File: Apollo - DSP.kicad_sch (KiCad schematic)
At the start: 27 parts, among them J1 USB_C_Receptacle_USB2.0, U1 NCP115ASN330T2G, U2 USBLC6-2SC6, U3 NCP115ASN330T2G

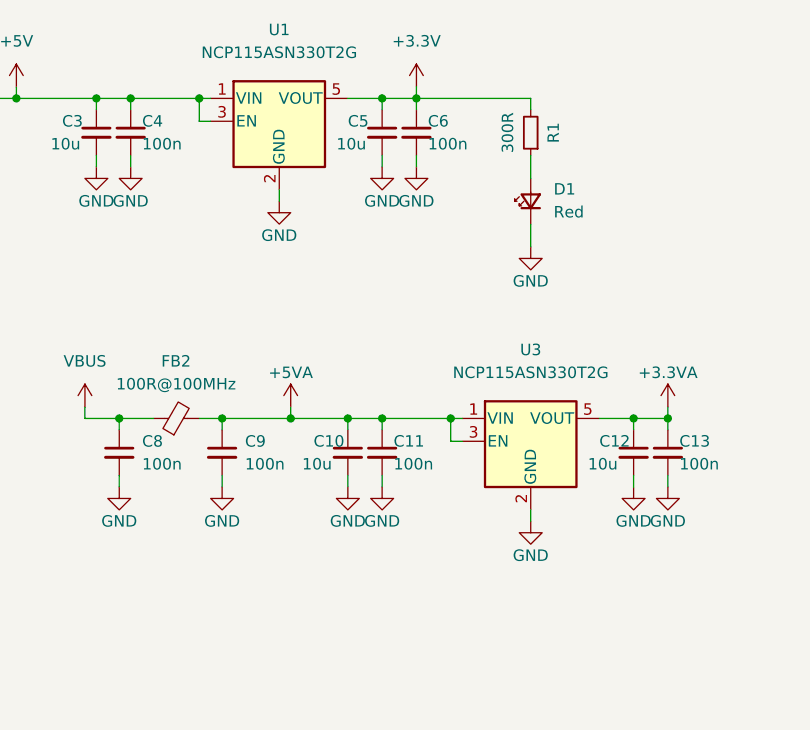
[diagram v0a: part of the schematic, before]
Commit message: own foorprint for LDO
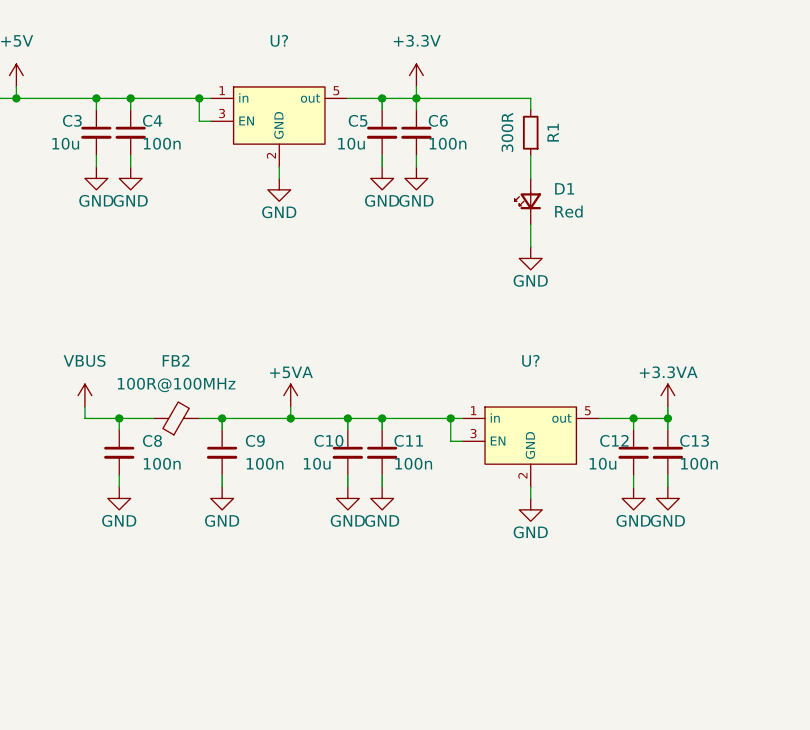
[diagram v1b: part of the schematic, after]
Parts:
- removed U1, U3: NCP115ASN330T2G, Package_TO_SOT_SMD:SOT-23-5, symbol Regulator_Linear:AP2127K-3.3
- added U? (x2): (no value), symbol NCP115ASN330T2G:NCP115ASN330T2G
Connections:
- net +3.3VA: now also U?.5 (out)
- net +3V3: now also U?.5 (out)
- net +5V: now also U?.1 (in), U?.3 (EN)
- net +5VA: now also U?.1 (in), U?.3 (EN)
- net GND: now also U?.2 (GND), U?.2 (GND)
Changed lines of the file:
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@@
     (stroke (width 0) (type default) (color 0 0 0 0))
   )
-  (wire (pts (xy 130.81 41.91) (xy 130.81 43.18))
+  (wire (pts (xy 130.81 39.37) (xy 130.81 40.64))
     (stroke (width 0) (type default) (color 0 0 0 0))
   )
@@
     (stroke (width 0) (type default) (color 0 0 0 0))
   )
-  (wire (pts (xy 158.75 77.47) (xy 158.75 78.74))
+  (wire (pts (xy 158.75 74.93) (xy 158.75 76.2))
     (stroke (width 0) (type default) (color 0 0 0 0))
   )
@@
     (pin "1")
     (pin "2")
-  )
-  (symbol (lib_id "Regulator_Linear:AP2127K-3.3") (at 158.75 69.85 0) (unit 1)
-    (in_bom yes) (on_board yes) (fields_autoplaced)
-    (property "Reference" "U3" (id 0) (at 158.75 59.69 0))
-    (property "Value" "NCP115ASN330T2G" (id 1) (at 158.75 62.23 0))
-    (property "Footprint" "Package_TO_SOT_SMD:SOT-23-5" (id 2) (at 158.75 61.595 0)
-      (effects (font (size 1.27 1.27)) hide)
-    )
-    (property "Datasheet" "https://www.onsemi.com/pdf/datasheet/ncp115-d.pdf" (id 3) (at 158.75 67.31 0)
-      (effects (font (size 1.27 1.27)) hide)
-    )
-    (pin "1")
-    (pin "2")
-    (pin "3")
-    (pin "4")
-    (pin "5")
   )
   (symbol (lib_id "power:GND") (at 142.24 74.93 0) (unit 1)
@@
     (pin "1")
   )
-  (symbol (lib_id "Regulator_Linear:AP2127K-3.3") (at 130.81 34.29 0) (unit 1)
-    (in_bom yes) (on_board yes) (fields_autoplaced)
-    (property "Reference" "U1" (id 0) (at 130.81 24.13 0))
-    (property "Value" "NCP115ASN330T2G" (id 1) (at 130.81 26.67 0))
-    (property "Footprint" "Package_TO_SOT_SMD:SOT-23-5" (id 2) (at 130.81 26.035 0)
-      (effects (font (size 1.27 1.27)) hide)
-    )
-    (property "Datasheet" "https://www.onsemi.com/pdf/datasheet/ncp115-d.pdf" (id 3) (at 130.81 31.75 0)
-      (effects (font (size 1.27 1.27)) hide)
-    )
-    (pin "1")
-    (pin "2")
-    (pin "3")
-    (pin "4")
-    (pin "5")
-  )
   (symbol (lib_id "power:+5V") (at 101.6 30.48 0) (unit 1)
     (in_bom yes) (on_board yes) (fields_autoplaced)
@@
     (pin "1")
     (pin "2")
+  )
+  (symbol (lib_id "NCP115ASN330T2G:NCP115ASN330T2G") (at 130.81 33.02 0) (unit 1)
+    (in_bom yes) (on_board yes) (fields_autoplaced)
+    (property "Reference" "U?" (id 0) (at 130.81 25.4 0))
+    (property "Value" "" (id 1) (at 130.81 27.94 0))
+    (property "Footprint" "" (id 2) (at 132.08 24.13 0)
+      (effects (font (size 1.27 1.27)) hide)
+    )
+    (property "Datasheet" "https://www.onsemi.com/pdf/datasheet/ncp115-d.pdf" (id 3) (at 130.81 21.59 0)
+      (effects (font (size 1.27 1.27)) hide)
+    )
+    (pin "1")
+    (pin "2")
+    (pin "3")
+    (pin "5")
   )
   (symbol (lib_id "power:GND") (at 90.17 39.37 0) (unit 1)
@@
     (pin "1")
   )
+  (symbol (lib_id "NCP115ASN330T2G:NCP115ASN330T2G") (at 158.75 68.58 0) (unit 1)
+    (in_bom yes) (on_board yes) (fields_autoplaced)
+    (property "Reference" "U?" (id 0) (at 158.75 60.96 0))
+    (property "Value" "" (id 1) (at 158.75 63.5 0))
+    (property "Footprint" "" (id 2) (at 160.02 59.69 0)
+      (effects (font (size 1.27 1.27)) hide)
+    )
+    (property "Datasheet" "https://www.onsemi.com/pdf/datasheet/ncp115-d.pdf" (id 3) (at 158.75 57.15 0)
+      (effects (font (size 1.27 1.27)) hide)
+    )
+    (pin "1")
+    (pin "2")
+    (pin "3")
+    (pin "5")
+  )
   (symbol (lib_id "Device:C_Small") (at 90.17 35.56 0) (unit 1)
     (in_bom yes) (on_board yes) (fields_autoplaced)
@@
     (pin "1")
   )
-  (symbol (lib_id "power:GND") (at 158.75 78.74 0) (unit 1)
-    (in_bom yes) (on_board yes)
-    (property "Reference" "#PWR0112" (id 0) (at 158.75 85.09 0)
-      (effects (font (size 1.27 1.27)) hide)
-    )
-    (property "Value" "GND" (id 1) (at 158.75 82.55 0))
-    (property "Footprint" "" (id 2) (at 158.75 78.74 0)
-      (effects (font (size 1.27 1.27)) hide)
-    )
-    (property "Datasheet" "" (id 3) (at 158.75 78.74 0)
+  (symbol (lib_id "power:GND") (at 158.75 76.2 0) (unit 1)
+    (in_bom yes) (on_board yes)
+    (property "Reference" "#PWR0112" (id 0) (at 158.75 82.55 0)
+      (effects (font (size 1.27 1.27)) hide)
+    )
+    (property "Value" "GND" (id 1) (at 158.75 80.01 0))
+    (property "Footprint" "" (id 2) (at 158.75 76.2 0)
+      (effects (font (size 1.27 1.27)) hide)
+    )
+    (property "Datasheet" "" (id 3) (at 158.75 76.2 0)
       (effects (font (size 1.27 1.27)) hide)
     )
@@
     (pin "2")
   )
-  (symbol (lib_id "power:GND") (at 130.81 43.18 0) (unit 1)
-    (in_bom yes) (on_board yes)
-    (property "Reference" "#PWR0116" (id 0) (at 130.81 49.53 0)
-      (effects (font (size 1.27 1.27)) hide)
-    )
-    (property "Value" "GND" (id 1) (at 130.81 46.99 0))
-    (property "Footprint" "" (id 2) (at 130.81 43.18 0)
-      (effects (font (size 1.27 1.27)) hide)
-    )
-    (property "Datasheet" "" (id 3) (at 130.81 43.18 0)
+  (symbol (lib_id "power:GND") (at 130.81 40.64 0) (unit 1)
+    (in_bom yes) (on_board yes)
+    (property "Reference" "#PWR0116" (id 0) (at 130.81 46.99 0)
+      (effects (font (size 1.27 1.27)) hide)
+    )
+    (property "Value" "GND" (id 1) (at 130.81 44.45 0))
+    (property "Footprint" "" (id 2) (at 130.81 40.64 0)
+      (effects (font (size 1.27 1.27)) hide)
+    )
+    (property "Datasheet" "" (id 3) (at 130.81 40.64 0)
       (effects (font (size 1.27 1.27)) hide)
     )
@@
       (reference "R12") (unit 1) (value "33R") (footprint "Resistor_SMD:R_0603_1608Metric_Pad0.98x0.95mm_HandSolder")
     )
-    (path "/29fc2250-c13d-4f92-82dc-4201bf9206dc"
-      (reference "U1") (unit 1) (value "NCP115ASN330T2G") (footprint "Package_TO_SOT_SMD:SOT-23-5")
-    )
     (path "/68e0c342-0593-4780-8f29-05b8479887ed"
       (reference "U2") (unit 1) (value "USBLC6-2SC6") (footprint "SnapEDA Library:SOT95P280X145-6N")
     )
-    (path "/162d0798-9fd6-4324-aa6e-7b20b4a56a99"
-      (reference "U3") (unit 1) (value "NCP115ASN330T2G") (footprint "Package_TO_SOT_SMD:SOT-23-5")
-    )
     (path "/65c41d2a-7921-40f6-8a66-43d43155f96a/e9cfdde6-7112-4587-8587-8eb874bda1d5"
       (reference "U4") (unit 1) (value "STM32F401RBTx") (footprint "Package_QFP:LQFP-64_10x10mm_P0.5mm")
@@
       (reference "U7") (unit 1) (value "23A256 - SRAM") (footprint "Package_SO:SOIC-8_3.9x4.9mm_P1.27mm")
     )
+    (path "/609c70f4-1479-4ca4-a93e-8230d97706fb"
+      (reference "U?") (unit 1) (value "NCP115ASN330T2G") (footprint "NCP115ASN330T2G:NCP115ASN330T2G")
+    )
+    (path "/ae0bc033-5ea1-4c90-ad13-904a827000a4"
+      (reference "U?") (unit 1) (value "NCP115ASN330T2G") (footprint "NCP115ASN330T2G:NCP115ASN330T2G")
+    )
     (path "/65c41d2a-7921-40f6-8a66-43d43155f96a/12a2e309-94ba-47b4-a076-bcf7f0bbcc58"
